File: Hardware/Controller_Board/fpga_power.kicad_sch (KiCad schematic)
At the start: 58 parts, among them U201 XC7A35T-CPG236

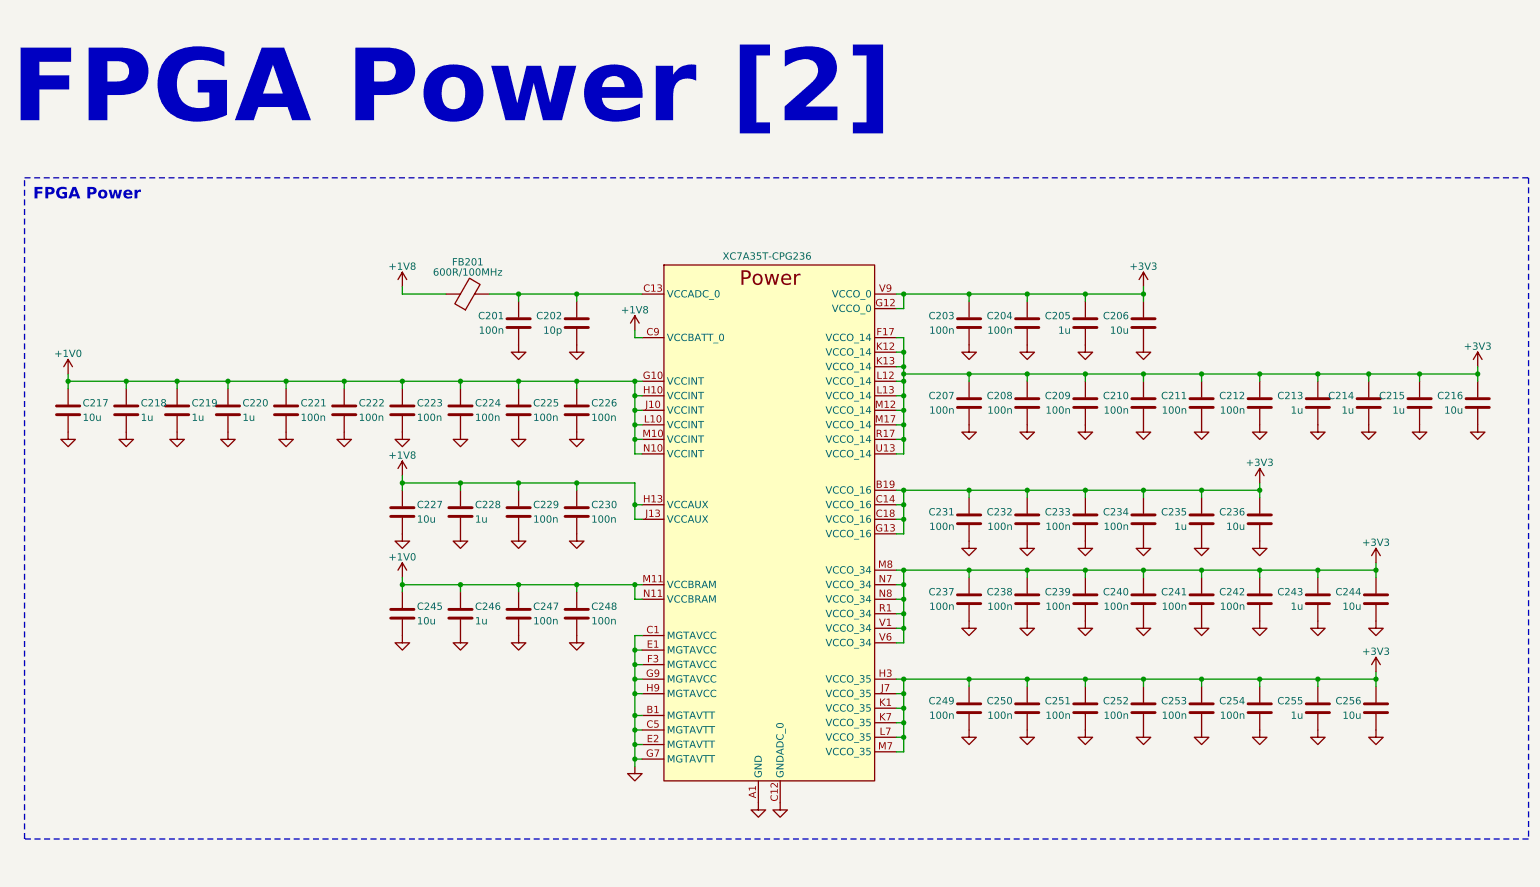
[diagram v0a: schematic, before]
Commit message: Started schematic rework and the PCB design
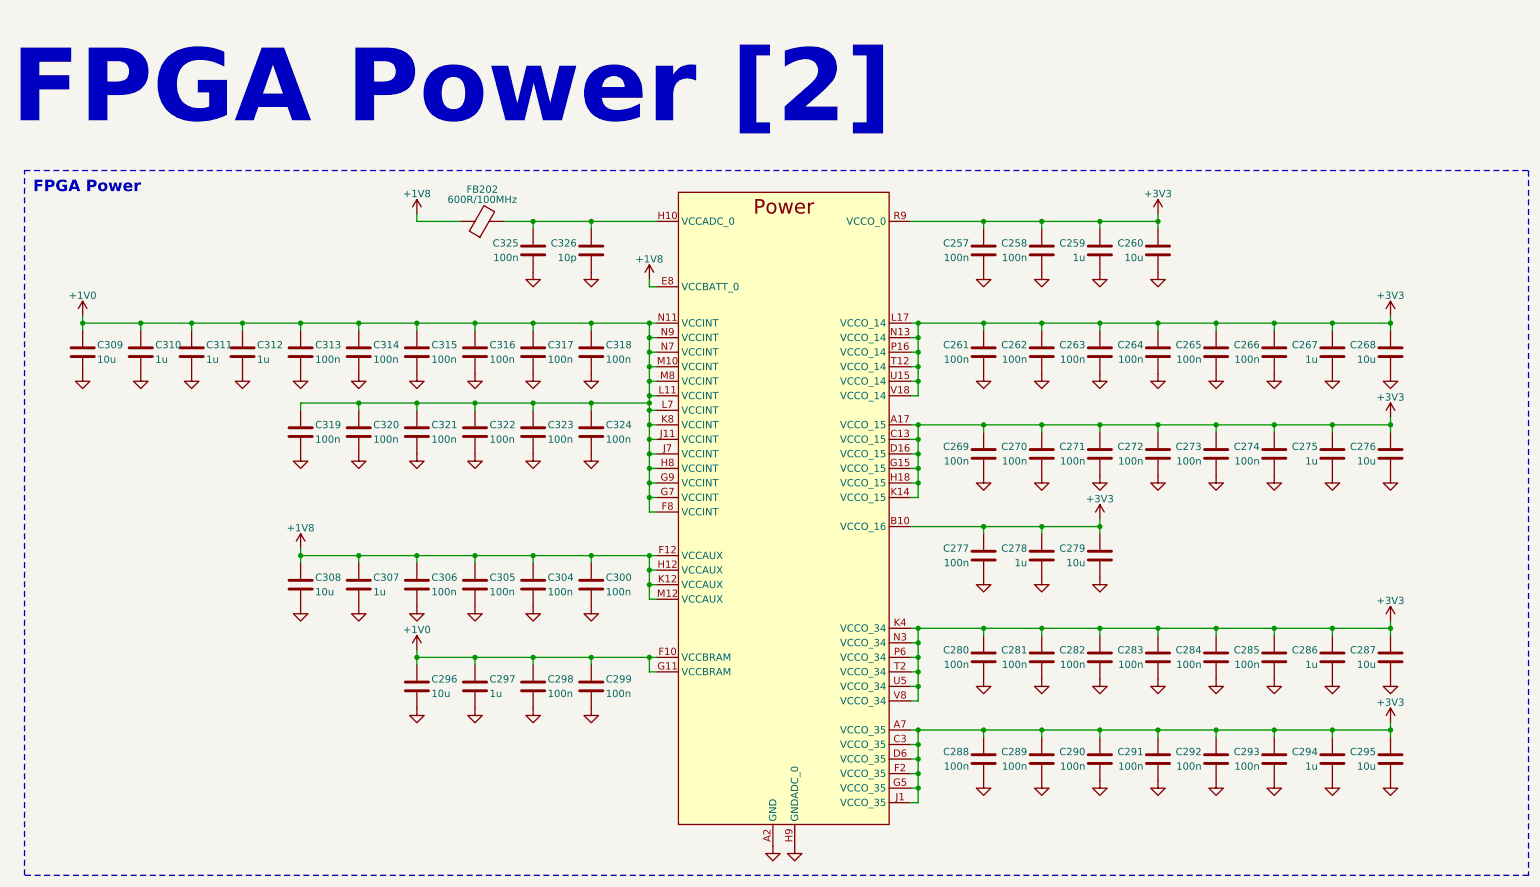
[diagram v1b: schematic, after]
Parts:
- removed C201: 100n, Capacitor_SMD:C_0402_1005Metric, symbol Device:C
- removed C202: 10p, Capacitor_SMD:C_0402_1005Metric, symbol Device:C
- removed C203, C204, C207, C208, C209, C210, C211, C212, C221, C222, C223, C224, C225, C226, C229, C230, C231, C232, C233, C234, C237, C238, C239, C240, C241, C242, C247, C248, C249, C250, C251, C252, C253, C254: 100n, Capacitor_SMD:C_0201_0603Metric, symbol Device:C
- removed C205, C213, C214, C215, C218, C219, C220, C228, C235, C243, C246, C255: 1u, Capacitor_SMD:C_0402_1005Metric, symbol Device:C
- removed C206, C216, C217, C227, C236, C244, C245, C256: 10u, Capacitor_SMD:C_0805_2012Metric, symbol Device:C
- removed FB201: 600R/100MHz, Inductor_SMD:L_0402_1005Metric, symbol Device:FerriteBead
- removed U201: XC7A35T-CPG236, Package_BGA:Xilinx_CPG236, symbol Custom_VoxLink_Symbols:XC7A35T-CPG236
- added C257, C258, C261, C262, C263, C264, C265, C266, C269, C270, C271, C272, C273, C274, C277, C280, C281, C282, C283, C284, C285, C288, C289, C290, C291, C292, C293, C298, C299, C300, C304, C305, C306, C313, C314, C315, C316, C317, C318, C319, C320, C321, C322, C323, C324: 100n, Capacitor_SMD:C_0201_0603Metric, symbol Device:C
- added C259, C267, C275, C278, C286, C294, C297, C307, C310, C311, C312: 1u, Capacitor_SMD:C_0402_1005Metric, symbol Device:C
- added C260, C268, C276, C279, C287, C295, C296, C308, C309: 10u, Capacitor_SMD:C_0805_2012Metric, symbol Device:C
- added C325: 100n, Capacitor_SMD:C_0402_1005Metric, symbol Device:C
- added C326: 10p, Capacitor_SMD:C_0402_1005Metric, symbol Device:C
- added FB202: 600R/100MHz, Inductor_SMD:L_0402_1005Metric, symbol Device:FerriteBead
- added U202: XC7A35T-CSG324, Package_BGA:Xilinx_CSG324, symbol Custom_VoxLink_Symbols:XC7A35T-CSG324
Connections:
- net +1V0: now also C296.1, C297.1, C298.1, C299.1, C309.1, C310.1, C311.1, C312.1, C313.1, C314.1, C315.1, C316.1, C317.1, C318.1, C319.1, C320.1, C321.1, C322.1, C323.1, C324.1, U202.F10 (VCCBRAM), U202.F8 (VCCINT), U202.G11 (VCCBRAM), U202.G7 (VCCINT), U202.G9 (VCCINT), U202.H8 (VCCINT), U202.J11 (VCCINT), U202.J7 (VCCINT), U202.K8 (VCCINT), U202.L11 (VCCINT), U202.L7 (VCCINT), U202.M10 (VCCINT), U202.M8 (VCCINT), U202.N11 (VCCINT), U202.N7 (VCCINT), U202.N9 (VCCINT)
- net +1V8: now also C300.1, C304.1, C305.1, C306.1, C307.1, C308.1, FB202.1, U202.E8 (VCCBATT_0), U202.F12 (VCCAUX), U202.H12 (VCCAUX), U202.K12 (VCCAUX), U202.M12 (VCCAUX)
- net +3V3: now also C257.1, C258.1, C259.1, C260.1, C261.1, C262.1, C263.1, C264.1, C265.1, C266.1, C267.1, C268.1, C269.1, C270.1, C271.1, C272.1, C273.1, C274.1, C275.1, C276.1, C277.1, C278.1, C279.1, C280.1, C281.1, C282.1, C283.1, C284.1, C285.1, C286.1, C287.1, C288.1, C289.1, C290.1, C291.1, C292.1, C293.1, C294.1, C295.1, U202.A17 (VCCO_15), U202.A7 (VCCO_35), U202.B10 (VCCO_16), U202.C13 (VCCO_15), U202.C3 (VCCO_35), U202.D16 (VCCO_15), U202.D6 (VCCO_35), U202.F2 (VCCO_35), U202.G15 (VCCO_15), U202.G5 (VCCO_35), U202.H18 (VCCO_15), U202.J1 (VCCO_35), U202.K14 (VCCO_15), U202.K4 (VCCO_34), U202.L17 (VCCO_14), U202.N13 (VCCO_14), U202.N3 (VCCO_34), U202.P16 (VCCO_14), U202.P6 (VCCO_34), U202.R9 (VCCO_0), U202.T12 (VCCO_14), U202.T2 (VCCO_34), U202.U15 (VCCO_14), U202.U5 (VCCO_34), U202.V18 (VCCO_14), U202.V8 (VCCO_34)
- net GND: now also C257.2, C258.2, C259.2, C260.2, C261.2, C262.2, C263.2, C264.2, C265.2, C266.2, C267.2, C268.2, C269.2, C270.2, C271.2, C272.2, C273.2, C274.2, C275.2, C276.2, C277.2, C278.2, C279.2, C280.2, C281.2, C282.2, C283.2, C284.2, C285.2, C286.2, C287.2, C288.2, C289.2, C290.2, C291.2, C292.2, C293.2, C294.2, C295.2, C296.2, C297.2, C298.2, C299.2, C300.2, C304.2, C305.2, C306.2, C307.2, C308.2, C309.2, C310.2, C311.2, C312.2, C313.2, C314.2, C315.2, C316.2, C317.2, C318.2, C319.2, C320.2, C321.2, C322.2, C323.2, C324.2, C325.2, C326.2, U202.A12 (GND), U202.A2 (GND), U202.B15 (GND), U202.B5 (GND), U202.C18 (GND), U202.C8 (GND), U202.D1 (GND), U202.D11 (GND), U202.E14 (GND), U202.E4 (GND), U202.F11 (GND), U202.F17 (GND), U202.F7 (GND), U202.F9 (GND), U202.G10 (GND), U202.G12 (GND), U202.G8 (GND), U202.H11 (GND), U202.H13 (GND), U202.H3 (GND), U202.H7 (GND), U202.H9 (GNDADC_0), U202.J12 (GND), U202.J16 (GND), U202.J6 (GND), U202.J8 (GND), U202.K11 (GND), U202.K7 (GND), U202.L12 (GND), U202.L2 (GND), U202.L8 (GND), U202.M11 (GND), U202.M15 (GND), U202.M5 (GND), U202.M7 (GND), U202.M9 (GND), U202.N10 (GND), U202.N12 (GND), U202.N18 (GND), U202.N8 (GND), U202.P1 (GND), U202.R14 (GND), U202.R4 (GND), U202.T17 (GND), U202.T7 (GND), U202.U10 (GND), U202.V13 (GND), U202.V3 (GND)
- new net: C325.1, C326.1, FB202.2, U202.H10 (VCCADC_0)
